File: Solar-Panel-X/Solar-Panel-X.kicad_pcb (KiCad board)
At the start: 6 copper layers, 48.4 x 48.4 mm, 81 parts, among them J1 FTS-105-01-L-DV-A, Q1 BSS138DWQ-7, Q2 MBT2222ADW1T1, Q3 BSS138DWQ-7, Q4 MBT2222ADW1T1, U1 BQ25570RGRR, U2 TSL2561

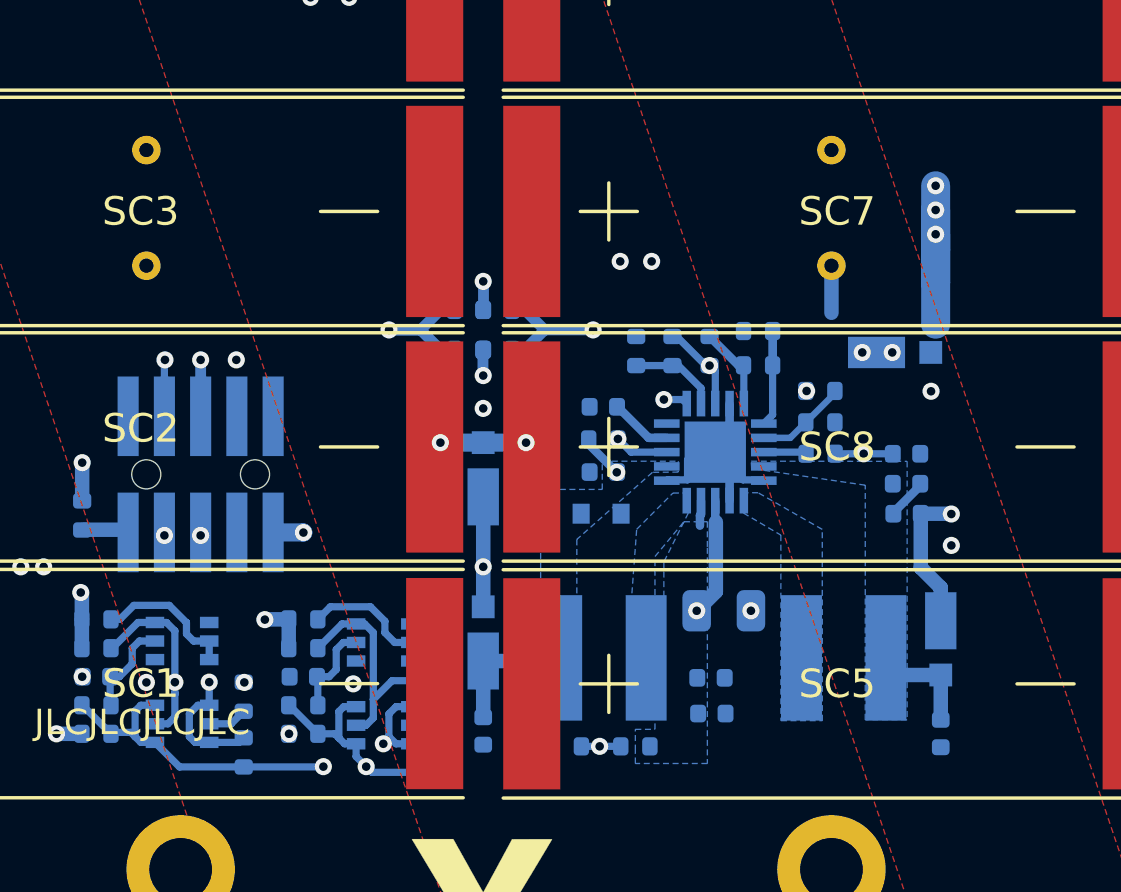
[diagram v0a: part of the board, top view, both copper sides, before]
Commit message: cleanup on X
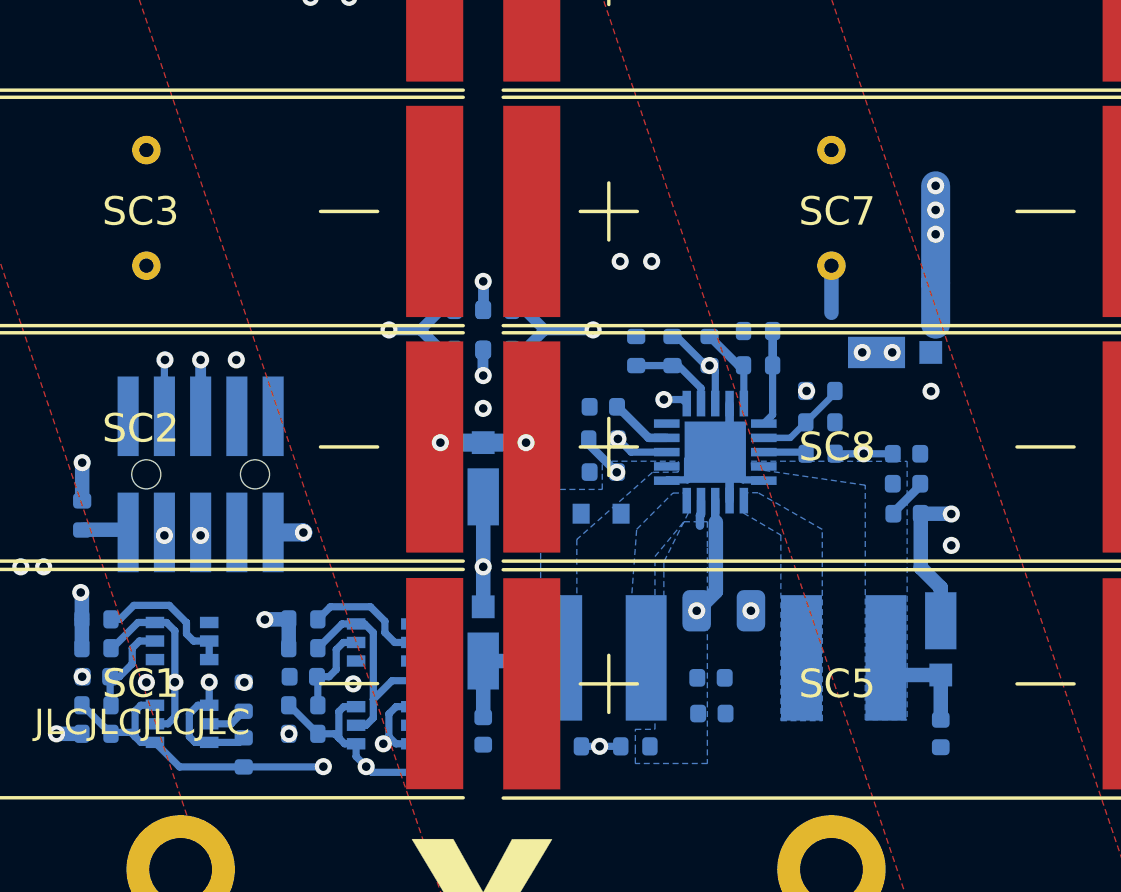
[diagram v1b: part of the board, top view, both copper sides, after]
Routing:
- net /coil: track 13208.5 -> 13203.6 mm
- net GND: track 28.3 -> 25.2 mm
- net Net-(D3-Pad1): track 14.4 -> 13.9 mm
